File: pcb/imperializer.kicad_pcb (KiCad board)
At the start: 2 copper layers, 85.1 x 99.1 mm, 24 parts, among them J1 USB_micro_horz_socket_reinfor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, J2 Conn_01x06_Male, SW1 SW_SPST, U1 AS1115-BSST, U2 ATMEGA32U4, U3 LTC-4727, U4 LTC-4727, U5 AP7313, X1 AVR_ISP, Y1 Resonator

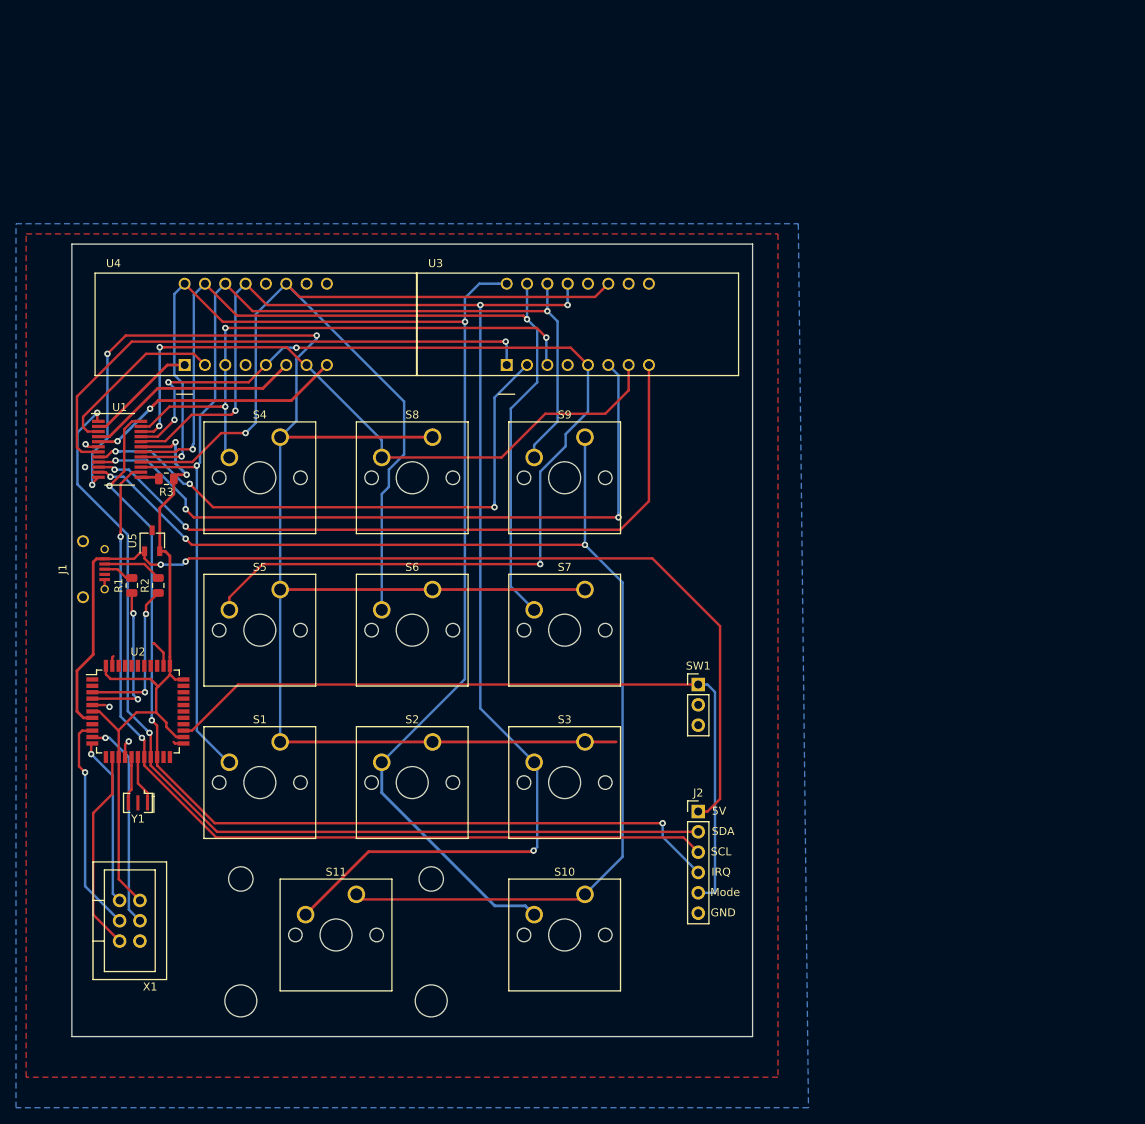
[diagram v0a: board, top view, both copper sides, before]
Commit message: pcb v1.1
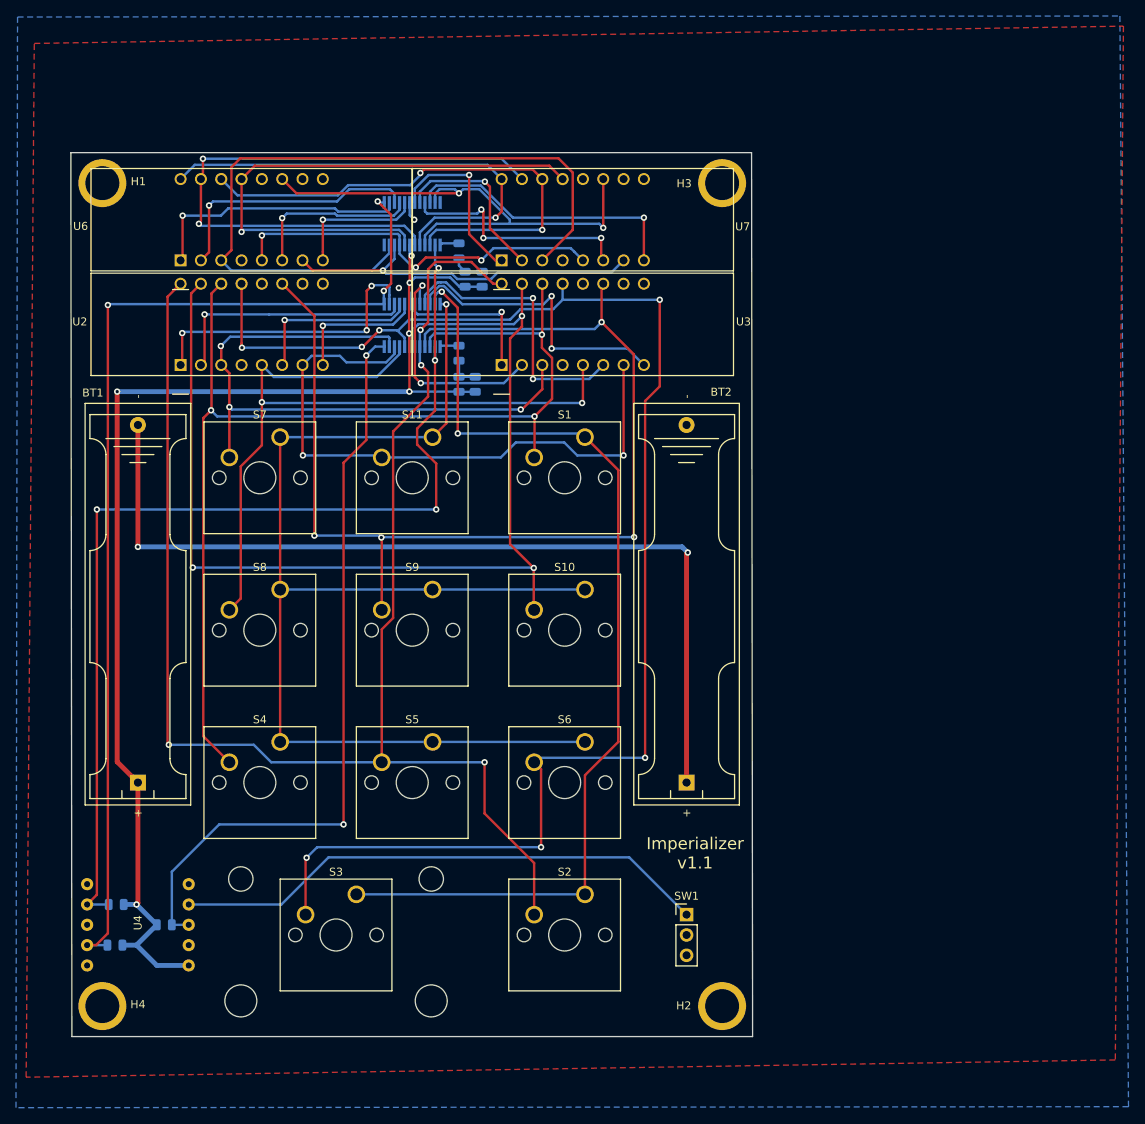
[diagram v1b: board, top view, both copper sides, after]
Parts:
- removed J1: USB_micro_horz_socket_reinforced, asl_footprints:microUSB_horizontal_socket
- removed J2: Conn_01x06_Male, Connector_PinHeader_2.54mm:PinHeader_1x06_P2.54mm_Vertical
- removed the S11 at (123.8, 118.1)
- removed U1: AS1115-BSST, Package_SO:QSOP-24_3.9x8.7mm_P0.635mm
- removed the U2 at (96.5, 95.2)
- removed X1: AVR_ISP, asl_footprints:AVR_ISP
- removed Y1: Resonator, Crystal:Resonator_SMD_muRata_CSTxExxV-3Pin_3.0x1.1mm
- added BT1: Battery, Battery:BatteryHolder_Keystone_2466_1xAAA, F.Cu at (96.5, 104.1)
- added BT2: Battery, Battery:BatteryHolder_Keystone_2466_1xAAA, F.Cu at (165.1, 104.1)
- added H1: Threaded_Standoff, asl_footprints:standoff_nut, F.Cu at (92.1, 29.2)
- added H2: Threaded_Standoff, asl_footprints:standoff_nut, F.Cu at (169.5, 132.1)
- added H3: Threaded_Standoff, asl_footprints:standoff_nut, F.Cu at (169.5, 29.2)
- added H4: Threaded_Standoff, asl_footprints:standoff_nut, F.Cu at (92.1, 132.1)
- added R4: 10KΩ, Resistor_SMD:R_0805_2012Metric, B.Cu at (136.7, 50.5)
- added R5: 10KΩ, Resistor_SMD:R_0805_2012Metric, B.Cu at (93.6, 124.5)
- added R6: 10KΩ, Resistor_SMD:R_0805_2012Metric, B.Cu at (93.8, 119.4)
- added R7: 10KΩ, Resistor_SMD:R_0805_2012Metric, B.Cu at (139.5, 41.2)
- added R8: 10KΩ, Resistor_SMD:R_0805_2012Metric, B.Cu at (137.4, 41.2)
- added R9: 10KΩ, Resistor_SMD:R_0805_2012Metric, B.Cu at (136.7, 37.7)
- added S6: switch_momentary_2pin, Button_Switch_Keyboard:SW_Cherry_MX_1.00u_PCB, F.Cu at (152.4, 99.1)
- added U4: trinket_M0, asl_footprints:trinket_M0, F.Cu at (96.5, 121.9)
- added U6: LTC-4727, asl_footprints:LTC-4727, F.Cu at (110.7, 33.8)
- added U7: LTC-4727, asl_footprints:LTC-4727, F.Cu at (150.9, 33.8)
- added U8: AS1115-BSST, Package_SO:QSOP-24_3.9x8.7mm_P0.635mm, B.Cu at (130.8, 34.3)
- R1, R2: value 27Ω -> 10KΩ; moved to B.Cu
- R3: value 25KΩ -> 10KΩ; moved to B.Cu
- S3: footprint Button_Switch_Keyboard:SW_Cherry_MX_1.00u_PCB -> Button_Switch_Keyboard:SW_Cherry_MX_2.00u_PCB
- U5: value AP7313 -> AS1115-BSST; footprint Package_TO_SOT_SMD:TSOT-23 -> Package_SO:QSOP-24_3.9x8.7mm_P0.635mm; moved to B.Cu
- moved R2 46.9 mm to (138.7, 54.4), turned to 270 degrees
- moved R1 42.6 mm to (99.8, 121.9), turned to 0 degrees
- moved U5 42.2 mm to (130.8, 47.0), turned to 270 degrees
- moved R3 38.4 mm to (136.7, 54.4), turned to 270 degrees
- moved S3 34.3 mm to (123.8, 118.1)
- moved SW1 28.8 mm to (165.1, 120.7)
- moved U3 0.63 mm to (150.9, 46.9)
- moved U2 0.51 mm to (110.7, 46.9)
- renumbered S9 to S1, S7 to S10, S8 to S11, S10 to S2, S1 to S4, S2 to S5, S4 to S7, S5 to S8, S6 to S9, U4 to U2
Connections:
- R1 pad 1: Net-(R1-Pad1) -> /VBATT
- R1 pad 2: Net-(J1-PadP3) -> /IRQ
- R2 pad 2: Net-(J1-PadP2) -> /VBATT
- R3 pad 1: /3.3VDC -> Net-(R2-Pad1)
- R3 pad 2: Net-(R3-Pad2) -> /VBATT
- S3 pad 1: /KEYB -> /KEYA
- U5 pad 1: /5VDC -> /SDA
- U5 pad 2: /3.3VDC -> /DIG0
- U5 pad 3: GND -> /DIG1
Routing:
- net /VBATT: track 0.00 -> 158.2 mm, vias 0 -> 6
- net /5VDC: track 130.7 -> 0.00 mm, vias 2 -> 0
- net Net-(BT1-Pad2): track 0.00 -> 113.1 mm, vias 0 -> 2
- net /d2: track 0.00 -> 92.0 mm
- net /3.3VDC: track 90.1 -> 0.00 mm, vias 2 -> 0
- net /g2: track 0.00 -> 78.0 mm, vias 0 -> 2
- net /c2: track 0.00 -> 70.1 mm, vias 0 -> 1
- net /f2: track 0.00 -> 66.4 mm, vias 0 -> 2
- net /a2: track 0.00 -> 64.8 mm, vias 0 -> 2
- net /b2: track 0.00 -> 58.5 mm, vias 0 -> 1
- net /DIG7: track 90.6 -> 37.1 mm
- net /DIG6: track 88.4 -> 35.8 mm, vias 3 -> 2
- net /DIG4: track 68.7 -> 18.7 mm
- net /e2: track 0.00 -> 48.3 mm, vias 0 -> 3
- net /KEYB: track 197.4 -> 151.4 mm, vias 3 -> 1
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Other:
- board size 85.1 x 99.1 mm -> 85.2 x 110.5 mm
- board text added: "Imperializer v1.1"
- board text removed: "5V"
- board text removed: "GND"
- board text removed: "IRQ"
- board text removed: "Mode"
- board text removed: "SCL"
- board text removed: "SDA"
